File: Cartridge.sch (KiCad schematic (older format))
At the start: 4 parts, among them J212 Diag, J24 Cartridge, J4 Expansion

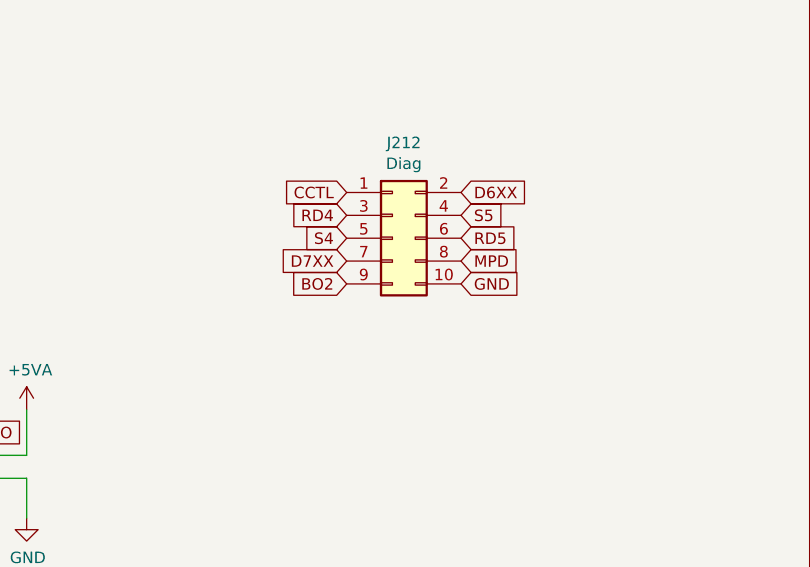
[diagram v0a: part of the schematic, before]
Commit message: Tracking
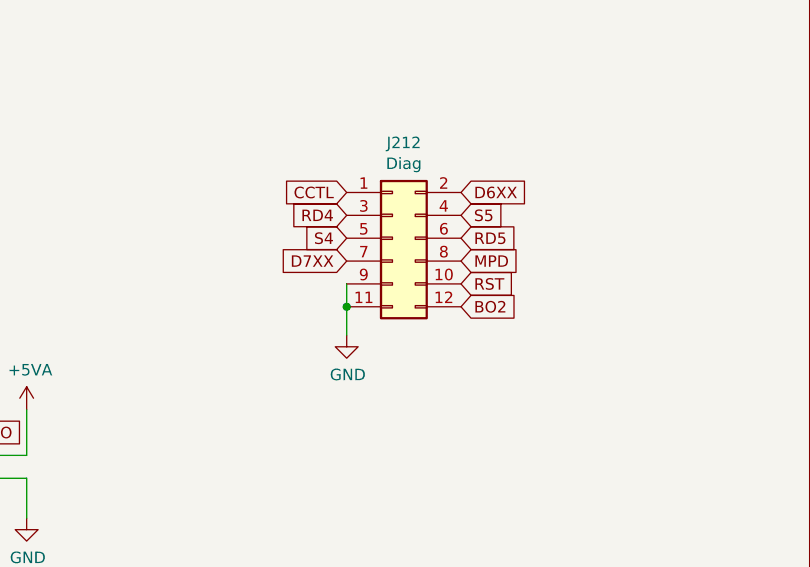
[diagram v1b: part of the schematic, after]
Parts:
- removed J212: Diag, Connector_PinHeader_2.54mm:PinHeader_2x05_P2.54mm_Vertical, symbol Connector_Generic:Conn_02x05_Odd_Even
- added J212: Diag, Connector_PinHeader_2.54mm:PinHeader_2x06_P2.54mm_Vertical, symbol Connector_Generic:Conn_02x06_Odd_Even
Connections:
- net BO2: now also J212.12 (Pin_12)
- net CCTL: now also J212.1 (Pin_1)
- net D6XX: now also J212.2 (Pin_2)
- net D7XX: now also J212.7 (Pin_7)
- net GND: now also J212.11 (Pin_11), J212.9 (Pin_9)
- net MPD: now also J212.8 (Pin_8)
- net RD4: now also J212.3 (Pin_3)
- net RD5: now also J212.6 (Pin_6)
- net RST: now also J212.10 (Pin_10)
- net S4: now also J212.5 (Pin_5)
- net S5: now also J212.4 (Pin_4)
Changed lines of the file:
@@
 Text GLabel 4525 3100 0    50   Input ~ 0
 D7XX
-Text GLabel 4525 3200 0    50   Input ~ 0
+Text GLabel 5025 3300 2    50   Input ~ 0
 BO2
 Text GLabel 4525 2800 0    50   Input ~ 0
@@
 D6XX
 Text GLabel 5025 3200 2    50   Input ~ 0
-GND
+RST
 Text GLabel 5025 3100 2    50   Input ~ 0
 MPD
 $Comp
-L Connector_Generic:Conn_02x05_Odd_Even J212
-U 1 1 604245DE
+L Connector_Generic:Conn_02x06_Odd_Even J212
+U 1 1 604B3554
 P 4725 3000
 F 0 "J212" H 4775 3417 50  0000 C CNN
 F 1 "Diag" H 4775 3326 50  0000 C CNN
-F 2 "Connector_PinHeader_2.54mm:PinHeader_2x05_P2.54mm_Vertical" H 4725 3000 50  0001 C CNN
+F 2 "Connector_PinHeader_2.54mm:PinHeader_2x06_P2.54mm_Vertical" H 4725 3000 50  0001 C CNN
 F 3 "~" H 4725 3000 50  0001 C CNN
 	1    4725 3000
 	1    0    0    -1
 $EndComp
+$Comp
+L power:GND #PWR?
+U 1 1 604B4D92
+P 4525 3425
+F 0 "#PWR?" H 4525 3175 50  0001 C CNN
+F 1 "GND" H 4530 3252 50  0000 C CNN
+F 2 "" H 4525 3425 50  0001 C CNN
+F 3 "" H 4525 3425 50  0001 C CNN
+	1    4525 3425
+	1    0    0    -1
+$EndComp
+Wire Wire Line
+	4525 3200 4525 3300
+Wire Wire Line
+	4525 3300 4525 3425
+Connection ~ 4525 3300
 $EndSCHEMATC
